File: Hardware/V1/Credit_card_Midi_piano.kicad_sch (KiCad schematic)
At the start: 11 parts, among them J101 MEM2085-00-115-00-A, J3 0, J4 0

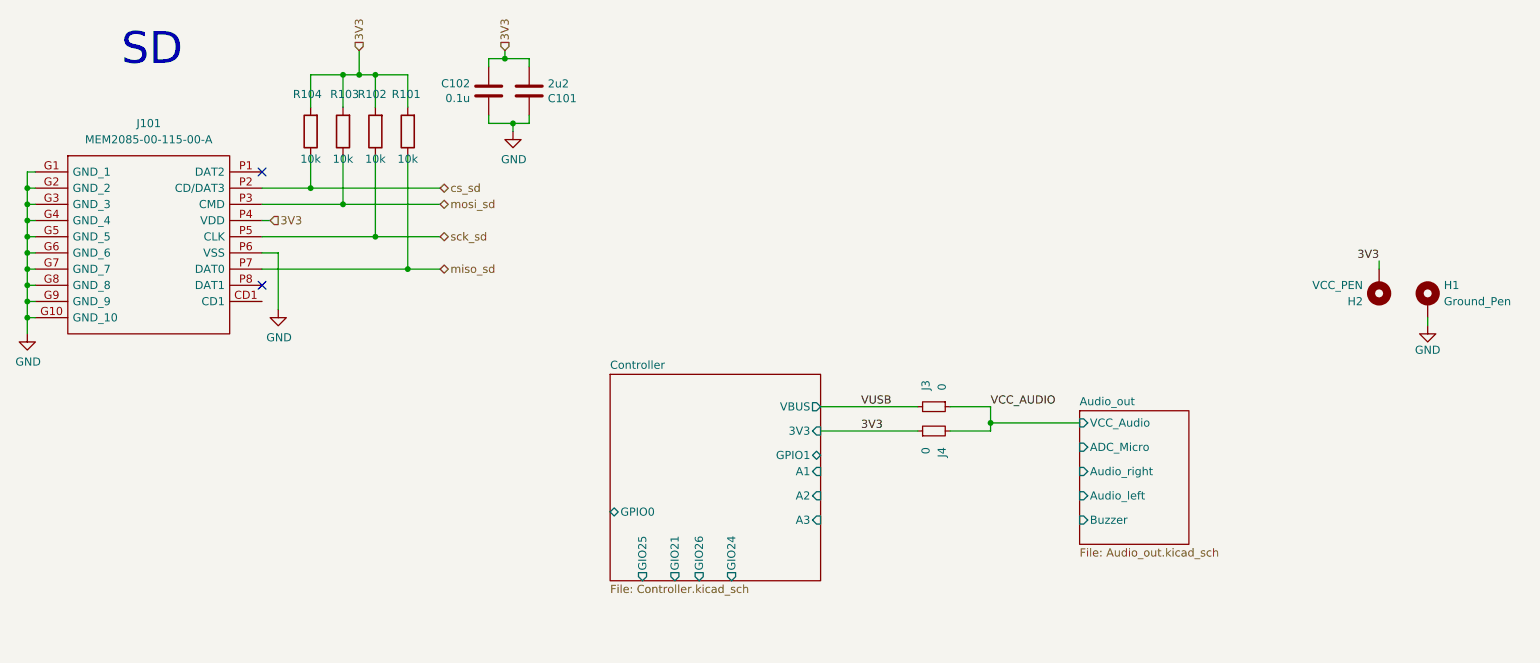
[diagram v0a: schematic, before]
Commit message: a
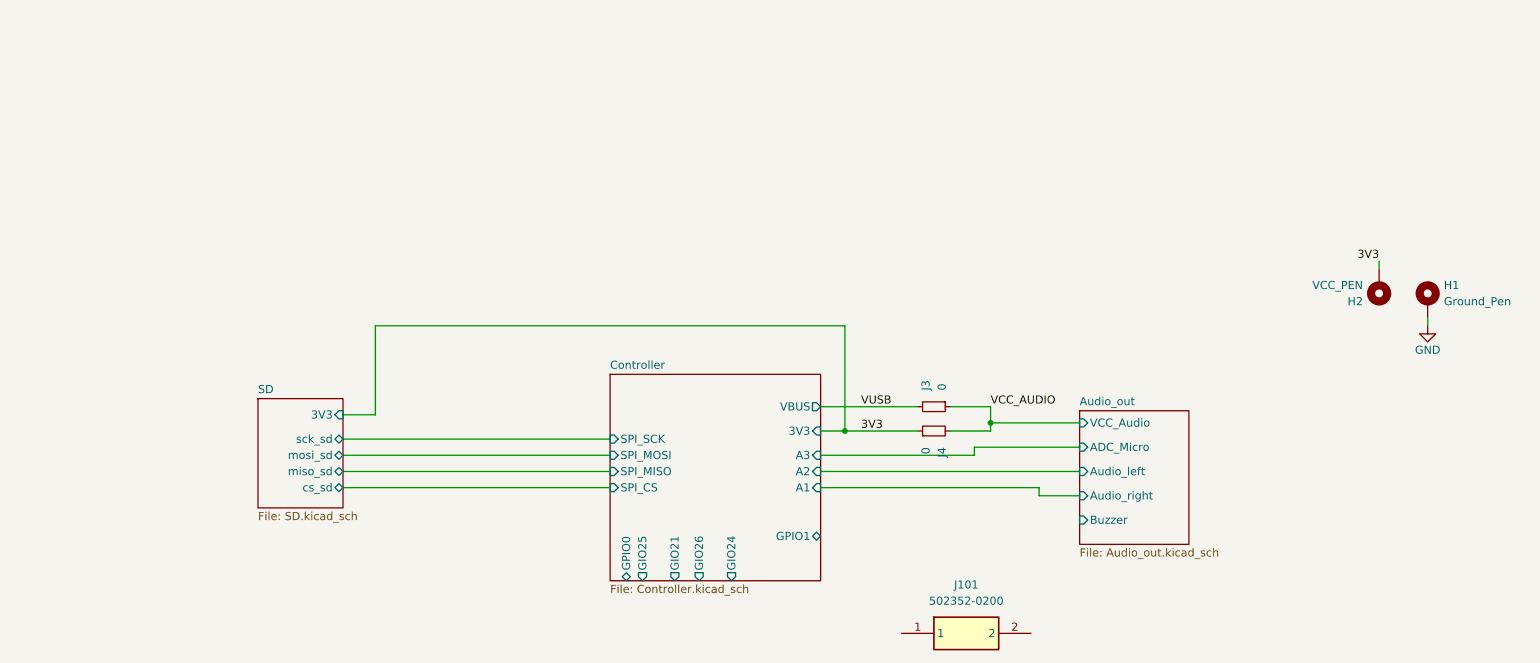
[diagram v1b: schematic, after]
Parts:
- removed C101: 2u2, Capacitor_SMD:C_0805_2012Metric_Pad1.18x1.45mm_HandSolder, symbol SymbolsBalloonv4:C
- removed C102: 0.1u, Capacitor_SMD:C_0402_1005Metric_Pad0.74x0.62mm_HandSolder, symbol SymbolsBalloonv4:C
- removed J101: MEM2085-00-115-00-A, SamacSys_Parts:MEM20850011500A, symbol SamacSys_Parts:MEM2085-00-115-00-A
- removed R101, R102, R103, R104: 10k, Resistor_SMD:R_0603_1608Metric_Pad0.98x0.95mm_HandSolder, symbol SymbolsBalloonv4:R
- added J101: 502352-0200, 5023520200, symbol SamacSys_Parts:502352-0200
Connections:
- no-connect marks 2 -> 0
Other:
- added sheet SD (SD.kicad_sch)
- sheet Controller ports: added SPI_CS, SPI_MISO, SPI_MOSI, SPI_SCK; removed none
- note removed: "SD"

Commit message: asd
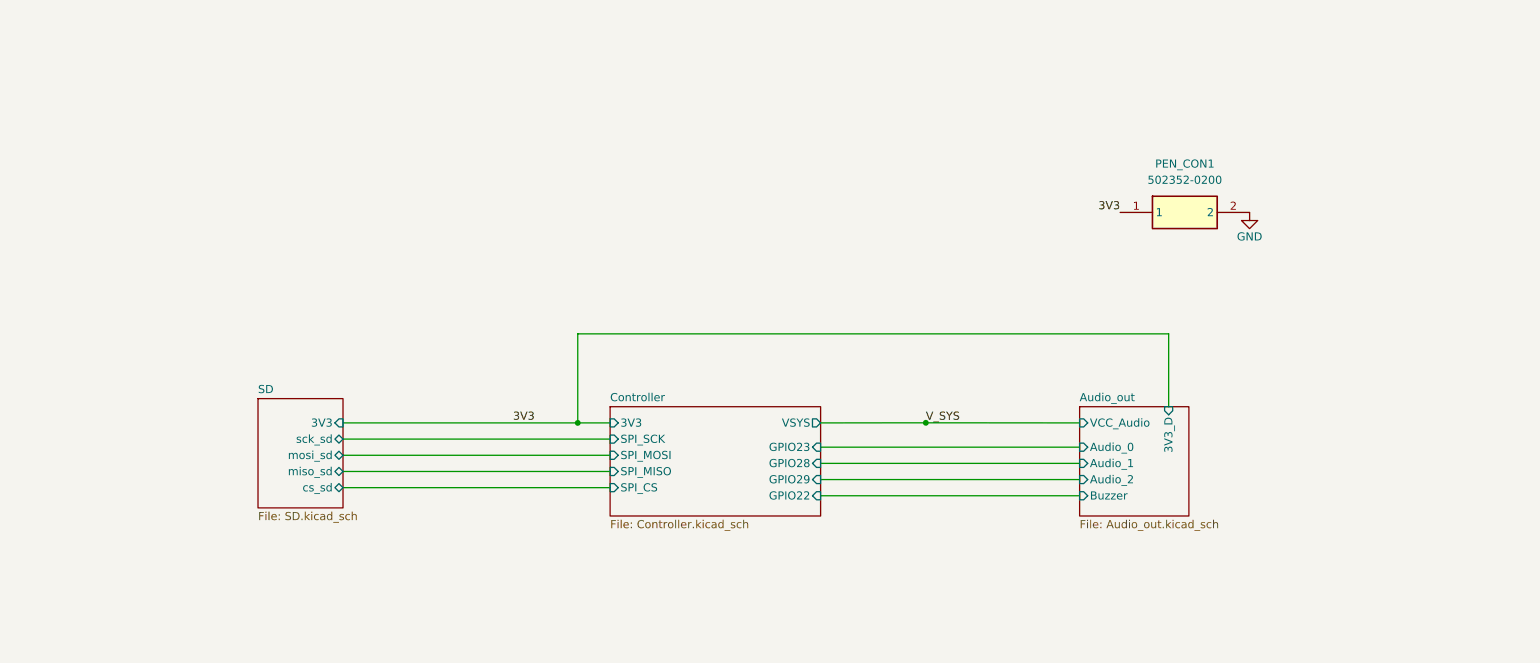
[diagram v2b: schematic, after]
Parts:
- removed H1: Ground_Pen, MountingHole:MountingHole_3.2mm_M3_Pad_Via, symbol Mechanical:MountingHole_Pad
- removed H2: VCC_PEN, MountingHole:MountingHole_3.2mm_M3_Pad_Via, symbol Mechanical:MountingHole_Pad
- removed J3, J4: 0, Resistor_SMD:R_0603_1608Metric, symbol Device:R_Small
- PEN_CON1: renamed from J101; footprint 5023520200 -> SamacSys_Parts:5023520200
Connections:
- net 3V3: now also PEN_CON1.1
- net GND: now also PEN_CON1.2
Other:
- sheet Audio_out ports: added 3V3_D, Audio_0, Audio_1, Audio_2; removed ADC_Micro, Audio_left, Audio_right
- sheet Controller ports: added GPIO22, GPIO23, GPIO28, GPIO29, VSYS; removed A1, A2, A3, GIO21, GIO24, GIO25, GIO26, GPIO0, GPIO1, VBUS
- moved on the sheet: PEN_CON1
